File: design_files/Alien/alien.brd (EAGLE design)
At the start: 20.7 x 24.6 mm, 6 parts

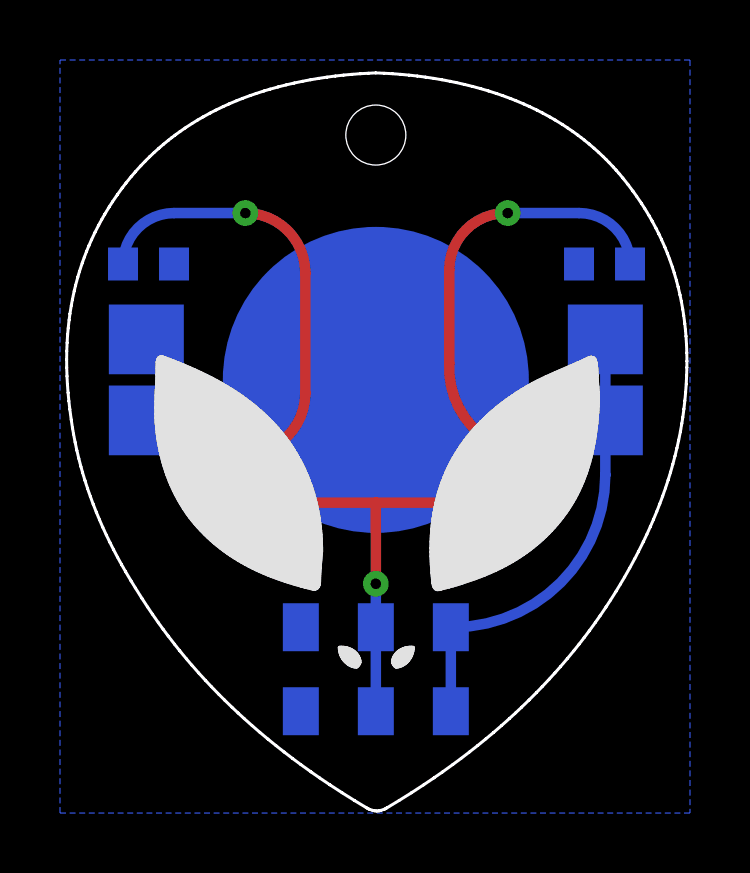
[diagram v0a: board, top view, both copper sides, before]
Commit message: adds updates and pics
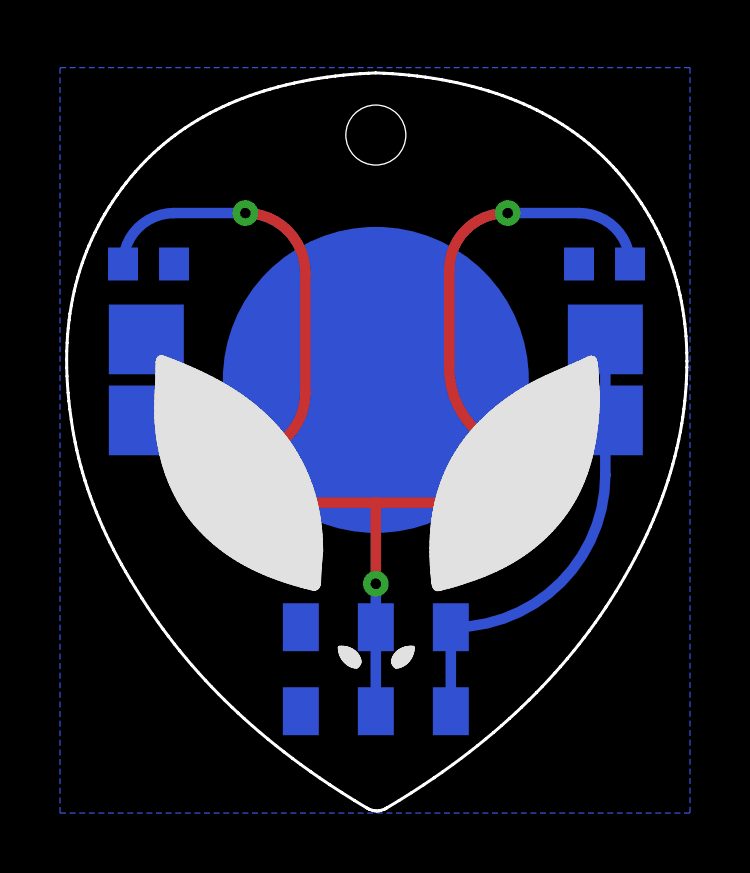
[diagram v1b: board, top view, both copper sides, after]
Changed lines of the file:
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@@
 <drawing>
 <settings>
-<setting alwaysvectorfont="yes"/>
+<setting alwaysvectorfont="no"/>
 <setting verticaltext="up"/>
 </settings>
@@
 </layers>
 <board>
-<fusionsync huburn="a.cGVyc29uYWw6dWUyYzY4MzUz" projecturn="a.cGVyc29uYWw6dWUyYzY4MzUzI0QyMDE5MDQwMzE4NjEyNjk4MQ" f3durn="urn:adsk.wipprod:dm.lineage:zyGNaZnlTEKXAFKFNzU47w" pcbguid="6b039789-e3a7-408c-8b21-c5d271b834b3" lastpulledtime="" lastsyncedchangeguid="089f73a4-3f89-014c-00c7-02fa9fe64186"/>
+<fusionsync huburn="a.cGVyc29uYWw6dWUyYzY4MzUz" projecturn="a.cGVyc29uYWw6dWUyYzY4MzUzI0QyMDE5MDQwMzE4NjEyNjk4MQ" f3durn="urn:adsk.wipprod:dm.lineage:zyGNaZnlTEKXAFKFNzU47w" pcbguid="6b039789-e3a7-408c-8b21-c5d271b834b3" lastpulledtime="" lastsyncedchangeguid="421bd0e0-7991-efe8-febd-e9999455af79"/>
 <plain>
 <wire x1="10.381759375" y1="0.067796875" x2="10.31265625" y2="0.073190625" width="0.1" layer="20"/>
@@
 </polygon>
 <hole x="10.35" y="22.6" drill="2"/>
+<dimension x1="20.8222" y1="0" x2="-0.1778" y2="0" x3="10.3222" y3="-0.0508" textsize="1.778" layer="1"/>
+<dimension x1="20.8222" y1="24.8476" x2="20.8222" y2="0" x3="-0.254" y3="12.4238" textsize="1.778" layer="1"/>
 </plain>
 <attributes>
@@
 <attribute name="VALUE" x="18.608" y="16.3966" size="1.27" layer="28" rot="MR0"/>
 </element>
-<element name="VBAT" library="SamacSys_Parts" package="BATHLD012SMT" override_package3d_urn="urn:adsk.eagle:package:15679619/3" override_package_urn="urn:adsk.eagle:footprint:15679620/1" override_locally_modified="yes" value="BAT-HLD-012-SMT" x="10.35" y="14.4386" smashed="yes" rot="MR0">
+<element name="VBAT" library="SamacSys_Parts" package="BATHLD012SMT" override_package3d_urn="urn:adsk.eagle:package:32568245/2" override_package_urn="urn:adsk.eagle:footprint:32568246/1" value="BAT-HLD-012-SMT" x="10.35" y="14.4386" smashed="yes" rot="MR0">
 <attribute name="DESCRIPTION" value="Coin Cell Battery Holders Bat Hld CR1216/1225 Surface Mount" x="10.35" y="14.4386" size="1.778" layer="28" rot="MR0" display="off"/>
 <attribute name="HEIGHT" value="3mm" x="10.35" y="14.4386" size="1.778" layer="28" rot="MR0" display="off"/>
@@
 <attribute name="MOUSER_PRICE-STOCK" value="https://www.mouser.com/Search/Refine.aspx?Keyword=712-BAT-HLD-012-SMT" x="10.35" y="14.4386" size="1.778" layer="28" rot="MR0" display="off"/>
 </element>
-<element name="U$1" library="electroninks" package="CL-SB-22A-02T-DPDT-COMPACT-SWITCH" override_package3d_urn="urn:adsk.eagle:package:15679591/3" override_package_urn="urn:adsk.eagle:footprint:15679592/1" value="CL-SB-22A-02T-SLIDE-SWITCH-TUCKED-PADS" x="10.35" y="4.7942" smashed="yes" rot="MR180"/>
+<element name="U$1" library="electroninks" package="CL-SB-22A-02T-DPDT-COMPACT-SWITCH" override_package3d_urn="urn:adsk.eagle:package:32568086/3" override_package_urn="urn:adsk.eagle:footprint:32568087/1" value="CL-SB-22A-02T-SLIDE-SWITCH-TUCKED-PADS" x="10.35" y="4.7942" smashed="yes" rot="MR180"/>
 </elements>
 <signals>
@@
 <contactref element="VBAT" pad="P$1"/>
 <polygon width="0.3048" layer="16">
-<vertex x="-0.1778" y="25.1016"/>
-<vertex x="20.8222" y="25.1016"/>
+<vertex x="-0.1778" y="24.8476"/>
+<vertex x="20.8222" y="24.8476"/>
 <vertex x="20.8222" y="0"/>
 <vertex x="-0.1778" y="0"/>
